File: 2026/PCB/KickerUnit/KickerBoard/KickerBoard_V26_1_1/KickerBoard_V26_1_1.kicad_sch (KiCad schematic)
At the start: 4 parts, among them Q1 FDS2582, T1 750032052, U1 LT3751UFD

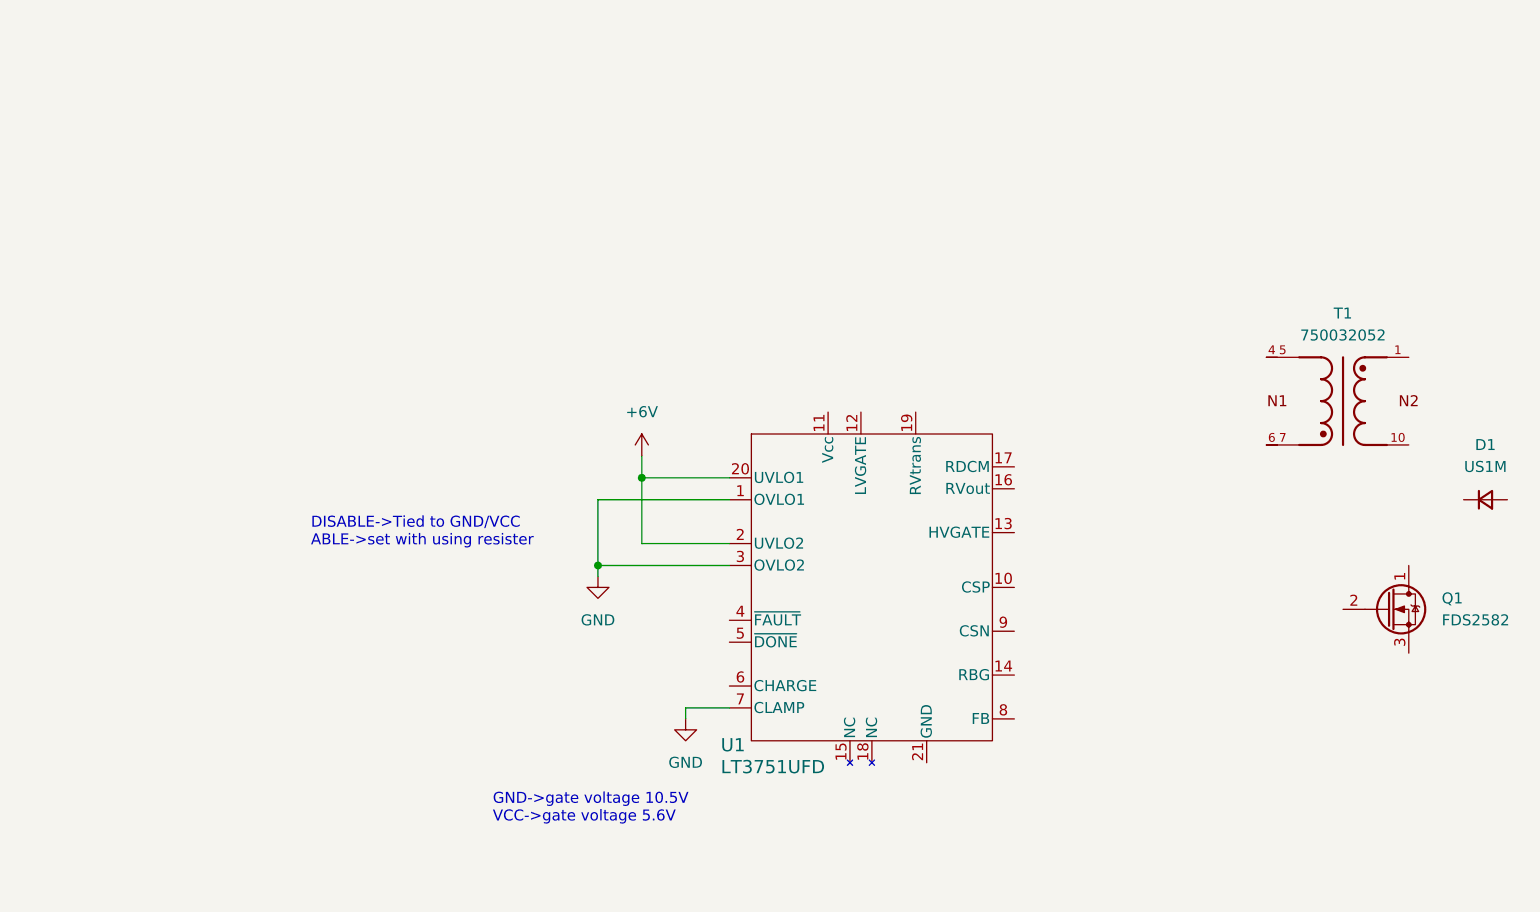
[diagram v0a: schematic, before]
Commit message: LT3751まわりの設計完了
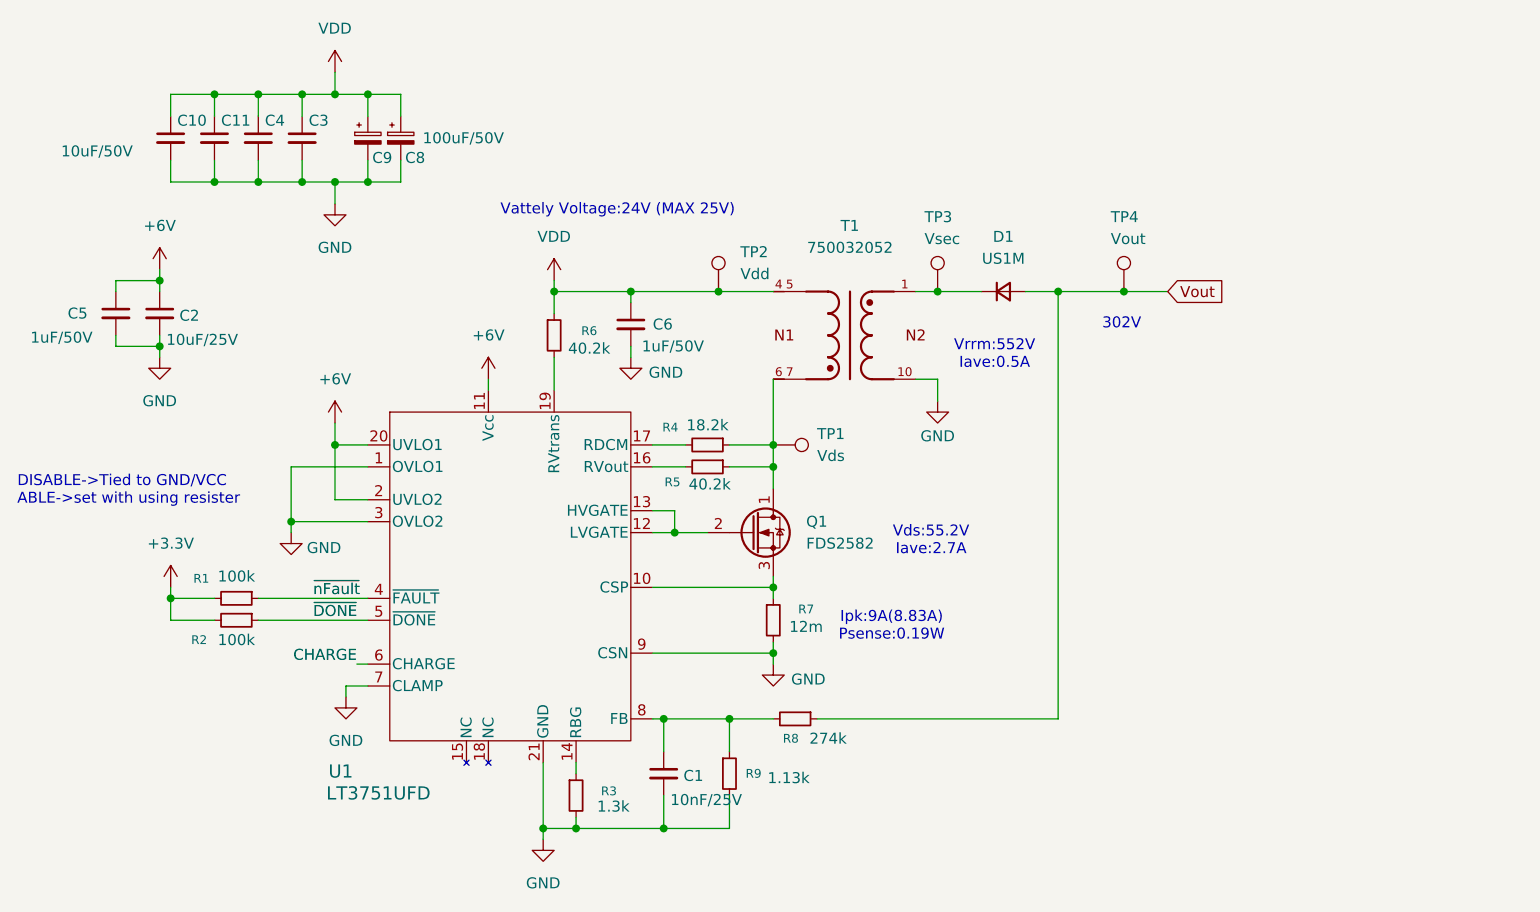
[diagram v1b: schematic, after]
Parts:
- added C1: 10nF/25V, symbol Device:C_Small
- added C10, C11, C3, C4: 10uF/50V, symbol Device:C_Small
- added C2: 10uF/25V, Resistor_SMD:R_0805_2012Metric_Pad1.20x1.40mm_HandSolder, symbol Device:C_Small
- added C5, C6: 1uF/50V, Resistor_SMD:R_0805_2012Metric_Pad1.20x1.40mm_HandSolder, symbol Device:C_Small
- added C8, C9: 100uF/50V, symbol Device:C_Polarized_Small
- added R1, R2: 100k, symbol Device:R_Small
- added R3: 1.3k, symbol Device:R_Small
- added R4: 18.2k, symbol Device:R_Small
- added R5, R6: 40.2k, symbol Device:R_Small
- added R7: 12m, Resistor_SMD:R_0805_2012Metric_Pad1.20x1.40mm_HandSolder, symbol Device:R_Small
- added R8: 274k, symbol Device:R_Small
- added R9: 1.13k, symbol Device:R_Small
- added TP1: Vds, symbol Connector:TestPoint
- added TP2: Vdd, symbol Connector:TestPoint
- added TP3: Vsec, symbol Connector:TestPoint
- added TP4: Vout, symbol Connector:TestPoint
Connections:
- net +6V: now also U1.11 (Vcc), C2.1, C5.1
- net GND: now also T1.10, U1.21 (GND), U1.9 (CSN), C1.2, C10.2, C11.2, C2.2, C3.2, C4.2, C5.2, C6.2, C8.2, C9.2, R3.2, R7.2, R9.2
- net at U1.10 (CSP): now also Q1.3 (S), R7.1
- net at U1.12 (LVGATE): now also Q1.2 (G), U1.13 (HVGATE)
- net at U1.14 (RBG): now also R3.1
- net at U1.16 (RVout): now also R5.2
- net at U1.17 (RDCM): now also R4.2
- net at U1.19 (RVtrans): now also R6.2
- net ~{nFault}: now reaches U1.4 (~{FAULT})
- net ~{nFault}: now also R1.1
- net ~{DONE}: now reaches U1.5 (~{DONE})
- net ~{DONE}: now also R2.1
- net CHARGE: now reaches U1.6 (CHARGE)
- net at U1.8 (FB): now also C1.1, R8.2, R9.1
- net at D1.1 (K): now also T1.1, TP3.1
- net Vout: now reaches D1.2 (A)
- net Vout: now also R8.1, TP4.1
- net at Q1.1 (D): now also T1.6, T1.7, R4.1, R5.1, TP1.1
- net VDD: now reaches T1.4, T1.5
- net VDD: now also C10.1, C11.1, C3.1, C4.1, C6.1, C8.1, C9.1, R6.1, TP2.1
- new net +3.3V: R1.2, R2.2
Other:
- note added: "302V"
- note added: "Ipk:9A(8.83A) Psense:0.19W"
- note added: "Vattely Voltage:24V (MAX 25V)"
- note added: "Vds:55.2V Iave:2.7A"
- note added: "Vrrm:552V Iave:0.5A"
- note removed: "GND->gate voltage 10.5V VCC->gate voltage 5.6V"
- moved on the sheet: D1, Q1, T1, U1
